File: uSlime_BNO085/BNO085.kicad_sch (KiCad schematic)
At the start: 13 parts, among them CN1 X1502WR-05K-N0SN, U1 BNO085

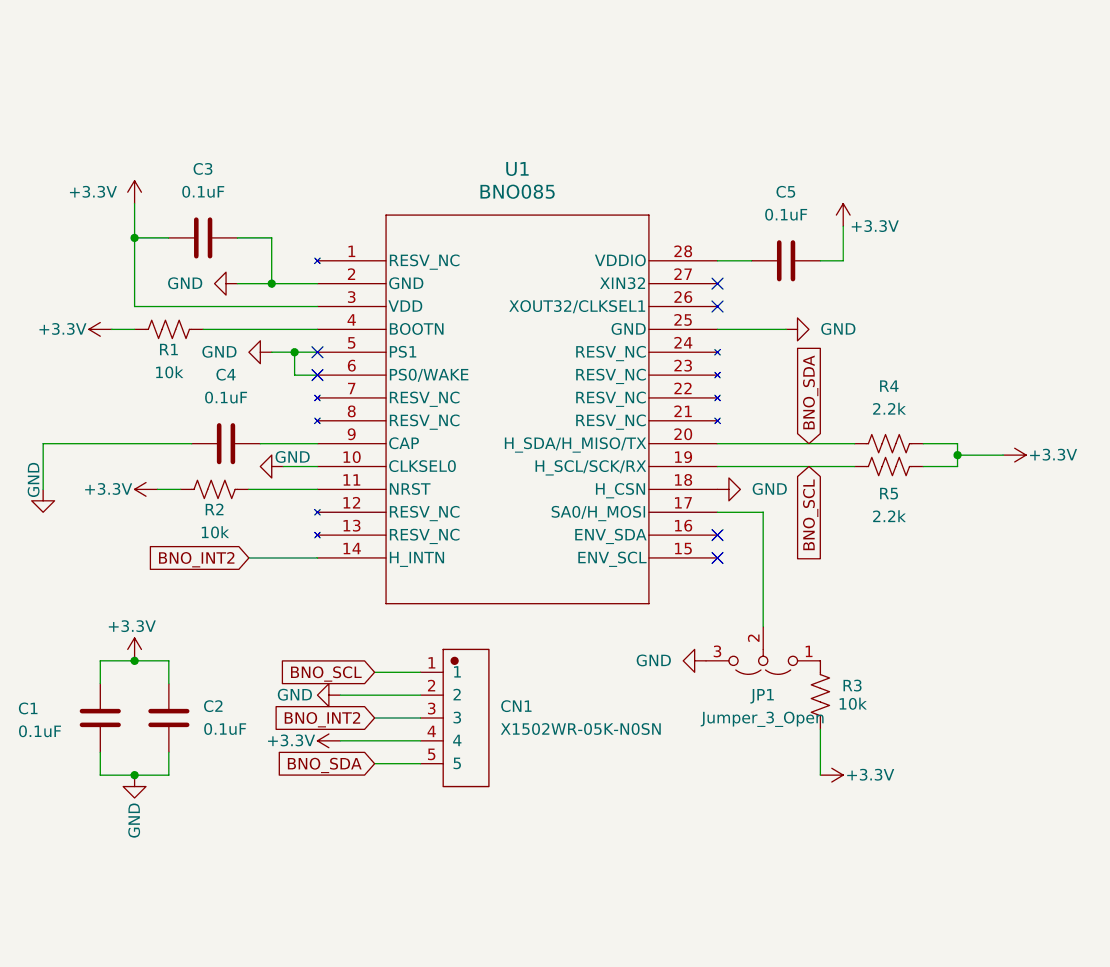
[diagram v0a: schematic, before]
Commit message: Update main PCB schematic
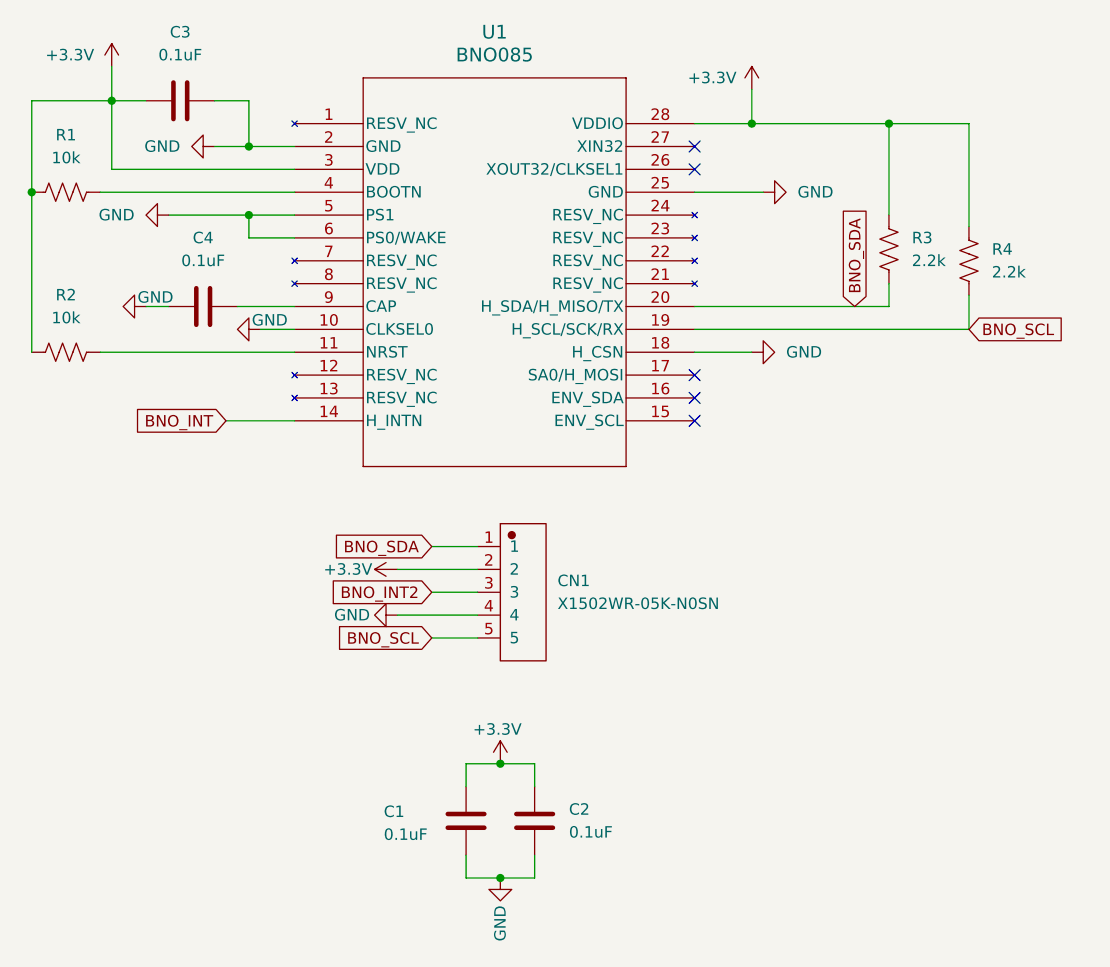
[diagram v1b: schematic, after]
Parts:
- removed C5: 0.1uF, Capacitor_SMD:C_0402_1005Metric, symbol uSlime:C
- removed JP1: Jumper_3_Open, Jumper:SolderJumper-3_P1.3mm_Open_RoundedPad1.0x1.5mm, symbol uSlime:Jumper_3_Open
- removed R5: 2.2k, Resistor_SMD:R_0402_1005Metric, symbol uSlime:R_US
- R3: value 10k -> 2.2k
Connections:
- net +3.3V: now also CN1.2, R2.2, R4.1, U1.28 (VDDIO); no longer CN1.4, R2.1, R4.2
- net BNO_INT2: no longer U1.14 (H_INTN)
- net BNO_SCL: now also CN1.5, R4.2; no longer CN1.1
- net BNO_SDA: now also CN1.1, R3.2; no longer CN1.5, R4.1
- net GND: now also CN1.4; no longer CN1.2
- net at U1.11 (NRST): now also R2.1; no longer R2.2
- new net BNO_INT: U1.14 (H_INTN)
- no-connect marks 6 -> 5
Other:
- moved on the sheet: C1, C2
